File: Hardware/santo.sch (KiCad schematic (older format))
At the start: 1 part

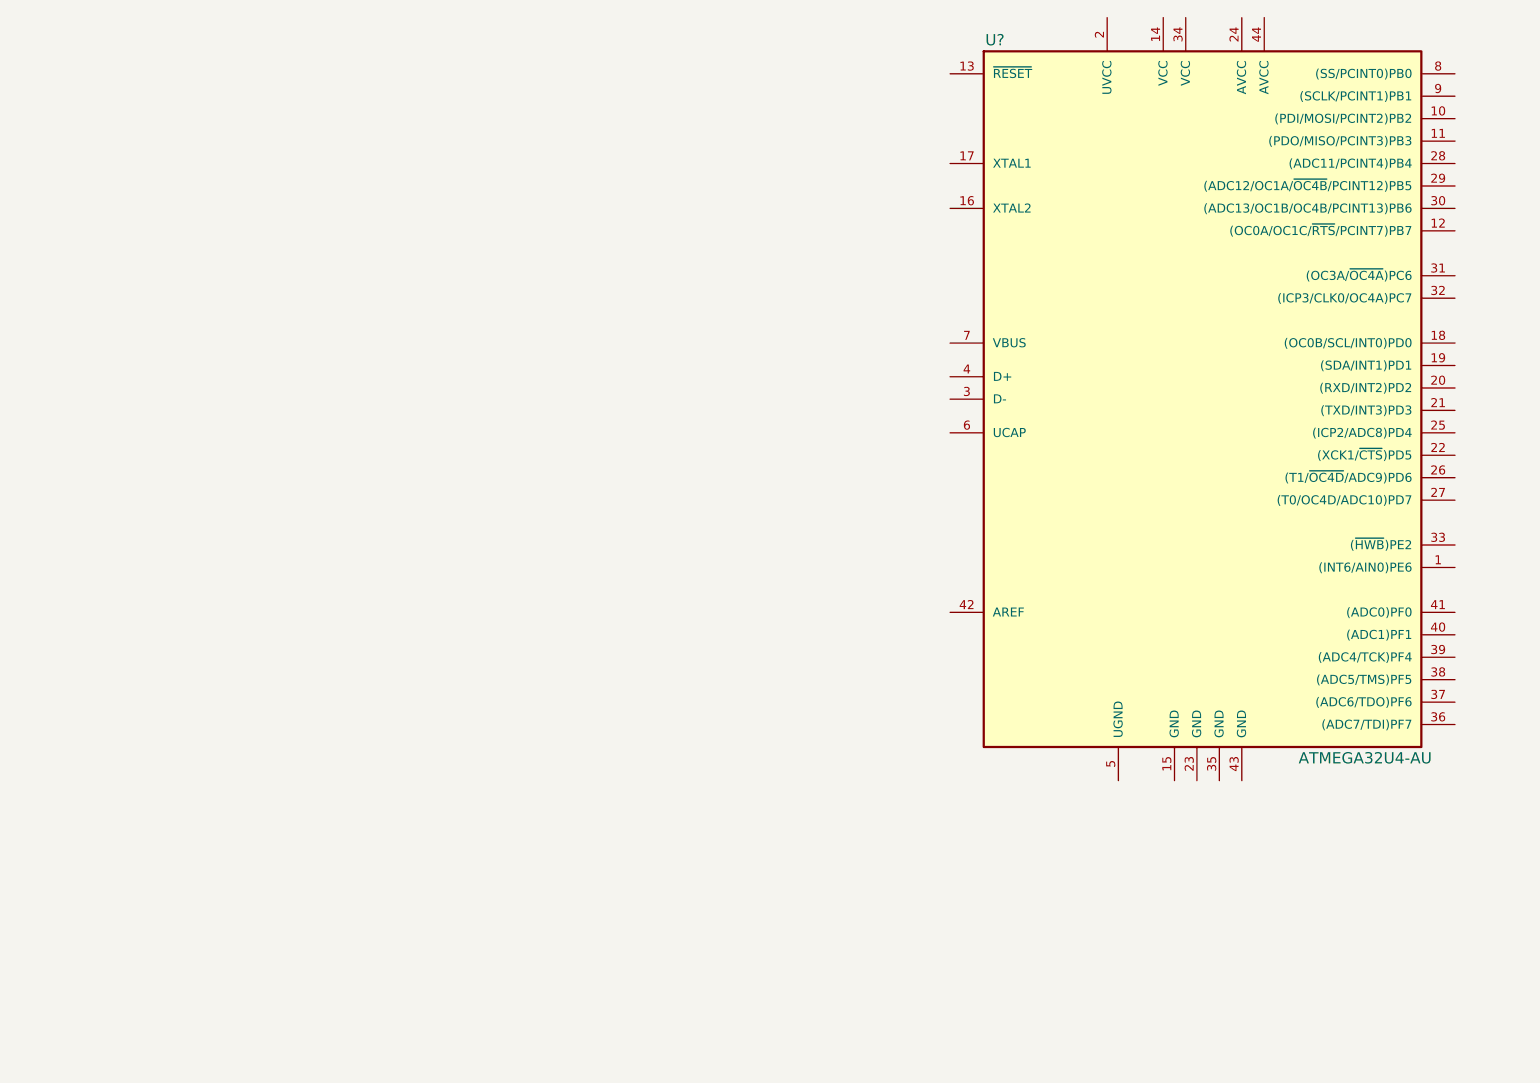
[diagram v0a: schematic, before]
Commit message: partial need to finish wiring up usb-c
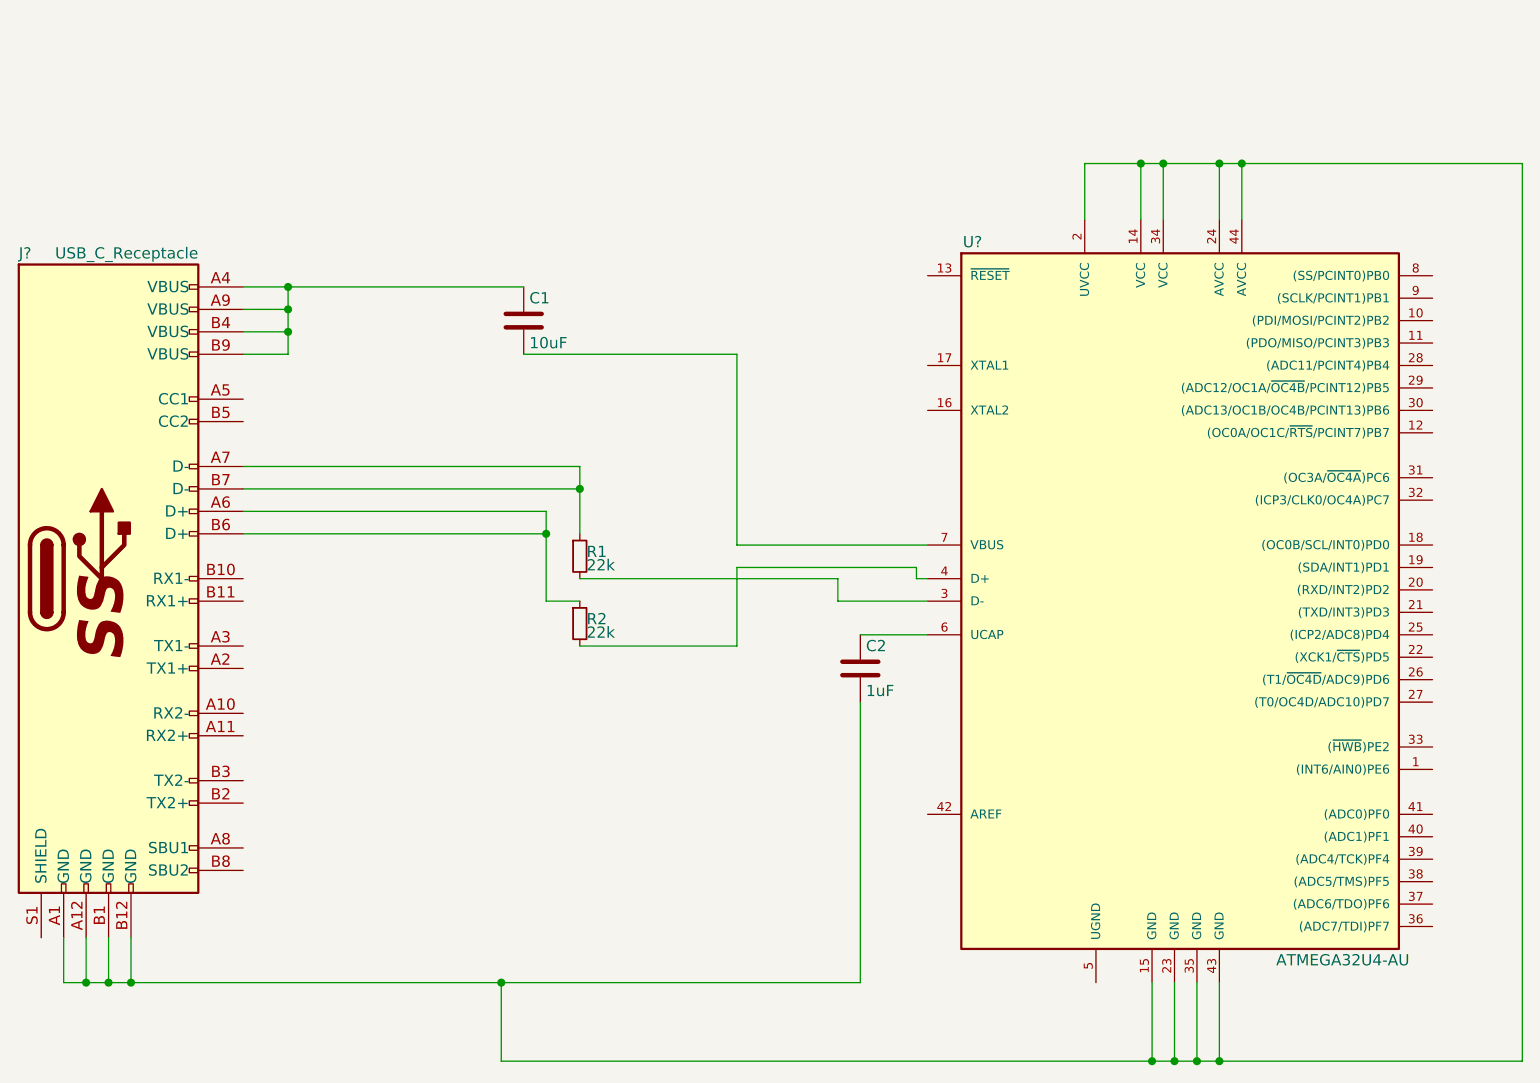
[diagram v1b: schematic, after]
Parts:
- added C1: 10uF, symbol C
- added C2: 1uF, symbol C
- added J?: USB_C_Receptacle, symbol USB_C_Receptacle
- added R1, R2: 22k, symbol R_Small
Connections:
- net at U?.14 (VCC): now also U?.15 (GND), U?.2 (UVCC), U?.23 (GND), U?.24 (AVCC), U?.34 (VCC), U?.35 (GND), U?.43 (GND), U?.44 (AVCC), C2.2, J?.A1 (GND), J?.A12 (GND), J?.B1 (GND), J?.B12 (GND)
- net at U?.3 (D-): now also R1.2
- net at U?.4 (D+): now also R2.2
- net at U?.6 (UCAP): now also C2.1
- net at U?.7 (VBUS): now also C1.2
- new net: C1.1, J?.A4 (VBUS), J?.A9 (VBUS), J?.B4 (VBUS), J?.B9 (VBUS)
- new net: J?.A6 (D+), J?.B6 (D+), R2.1
- new net: J?.A7 (D-), J?.B7 (D-), R1.1
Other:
- moved on the sheet: U?
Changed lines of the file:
@@
 LIBS:contrib
 LIBS:valves
+LIBS:santo-cache
 EELAYER 25 0
 EELAYER END
@@
 L ATMEGA32U4-AU U?
 U 1 1 59F3E9EC
-P 5900 3450
-F 0 "U?" H 4950 5150 50  0000 C CNN
-F 1 "ATMEGA32U4-AU" H 6600 1950 50  0000 C CNN
-F 2 "TQFP44" H 5900 3450 50  0001 C CIN
-F 3 "" H 7000 4550 50  0001 C CNN
-	1    5900 3450
+P 5800 4350
+F 0 "U?" H 4850 6050 50  0000 C CNN
+F 1 "ATMEGA32U4-AU" H 6500 2850 50  0000 C CNN
+F 2 "TQFP44" H 5800 4350 50  0001 C CIN
+F 3 "" H 6900 5450 50  0001 C CNN
+	1    5800 4350
 	1    0    0    -1
 $EndComp
+$Comp
+L USB_C_Receptacle J?
+U 1 1 59F5288B
+P 1000 4150
+F 0 "J?" H 600 5600 50  0000 L CNN
+F 1 "USB_C_Receptacle" H 1400 5600 50  0000 R CNN
+F 2 "" H 1150 4150 50  0001 C CNN
+F 3 "" H 1150 4150 50  0001 C CNN
+	1    1000 4150
+	1    0    0    -1
+$EndComp
+Wire Wire Line
+	1600 2950 1800 2950
+Wire Wire Line
+	1800 2850 1800 3150
+Connection ~ 1800 2850
+Wire Wire Line
+	1800 3050 1600 3050
+Connection ~ 1800 2950
+Wire Wire Line
+	1800 3150 1600 3150
+Connection ~ 1800 3050
+$Comp
+L R_Small R2
+U 1 1 59F52DAB
+P 3100 4350
+F 0 "R2" H 3130 4370 50  0000 L CNN
+F 1 "22k" H 3130 4310 50  0000 L CNN
+F 2 "" H 3100 4350 50  0001 C CNN
+F 3 "" H 3100 4350 50  0001 C CNN
+	1    3100 4350
+	1    0    0    -1
+$EndComp
+$Comp
+L R_Small R1
+U 1 1 59F52DD6
+P 3100 4050
+F 0 "R1" H 3130 4070 50  0000 L CNN
+F 1 "22k" H 3130 4010 50  0000 L CNN
+F 2 "" H 3100 4050 50  0001 C CNN
+F 3 "" H 3100 4050 50  0001 C CNN
+	1    3100 4050
+	1    0    0    -1
+$EndComp
+Wire Wire Line
+	1600 3650 3100 3650
+Wire Wire Line
+	3100 3650 3100 3950
+Wire Wire Line
+	1600 3750 3100 3750
+Connection ~ 3100 3750
+Wire Wire Line
+	3100 4150 4250 4150
+Wire Wire Line
+	4250 4150 4250 4250
+Wire Wire Line
+	4250 4250 4650 4250
+Wire Wire Line
+	1600 3850 2950 3850
+Wire Wire Line
+	2950 3850 2950 4250
+Wire Wire Line
+	2950 4250 3100 4250
+Wire Wire Line
+	1600 3950 2950 3950
+Connection ~ 2950 3950
+Wire Wire Line
+	3100 4450 3800 4450
+Wire Wire Line
+	3800 4450 3800 4100
+Wire Wire Line
+	3800 4100 4600 4100
+Wire Wire Line
+	4600 4100 4600 4150
+Wire Wire Line
+	4600 4150 4650 4150
+Wire Wire Line
+	1600 2850 2850 2850
+$Comp
+L C C1
+U 1 1 59F5311D
+P 2850 3000
+F 0 "C1" H 2875 3100 50  0000 L CNN
+F 1 "10uF" H 2875 2900 50  0000 L CNN
+F 2 "" H 2888 2850 50  0001 C CNN
+F 3 "" H 2850 3000 50  0001 C CNN
+	1    2850 3000
+	1    0    0    -1
+$EndComp
+Wire Wire Line
+	2850 3150 3800 3150
+Wire Wire Line
+	3800 3150 3800 4000
+Wire Wire Line
+	3800 4000 4650 4000
+$Comp
+L C C2
+U 1 1 59F532C4
+P 4350 4550
+F 0 "C2" H 4375 4650 50  0000 L CNN
+F 1 "1uF" H 4375 4450 50  0000 L CNN
+F 2 "" H 4388 4400 50  0001 C CNN
+F 3 "" H 4350 4550 50  0001 C CNN
+	1    4350 4550
+	1    0    0    -1
+$EndComp
+Wire Wire Line
+	4350 4400 4650 4400
+Wire Wire Line
+	4350 4700 4350 5950
+Wire Wire Line
+	4350 5950 800  5950
+Wire Wire Line
+	800  5950 800  5750
+Wire Wire Line
+	900  5750 900  5950
+Connection ~ 900  5950
+Wire Wire Line
+	1000 5750 1000 5950
+Connection ~ 1000 5950
+Wire Wire Line
+	1100 5750 1100 5950
+Connection ~ 1100 5950
+Wire Wire Line
+	5350 2550 5350 2300
+Wire Wire Line
+	5350 2300 7300 2300
+Wire Wire Line
+	7300 2300 7300 6300
+Wire Wire Line
+	7300 6300 2750 6300
+Wire Wire Line
+	2750 6300 2750 5950
+Connection ~ 2750 5950
+Wire Wire Line
+	5600 2550 5600 2300
+Connection ~ 5600 2300
+Wire Wire Line
+	5700 2550 5700 2300
+Connection ~ 5700 2300
+Wire Wire Line
+	5950 2550 5950 2300
+Connection ~ 5950 2300
+Wire Wire Line
+	6050 2550 6050 2300
+Connection ~ 6050 2300
+Wire Wire Line
+	5650 5950 5650 6300
+Connection ~ 5650 6300
+Wire Wire Line
+	5750 5950 5750 6300
+Connection ~ 5750 6300
+Wire Wire Line
+	5850 5950 5850 6300
+Connection ~ 5850 6300
+Wire Wire Line
+	5950 5950 5950 6300
+Connection ~ 5950 6300
 $EndSCHEMATC
